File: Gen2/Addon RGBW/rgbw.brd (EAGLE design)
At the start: 59.4 x 48 mm, 33 parts, among them Q1 BUZ11, Q2 BUZ11, Q3 BUZ11, Q4 BUZ11, Q5 BUZ11, Q6 BUZ11, Q7 BUZ11, Q8 BUZ11

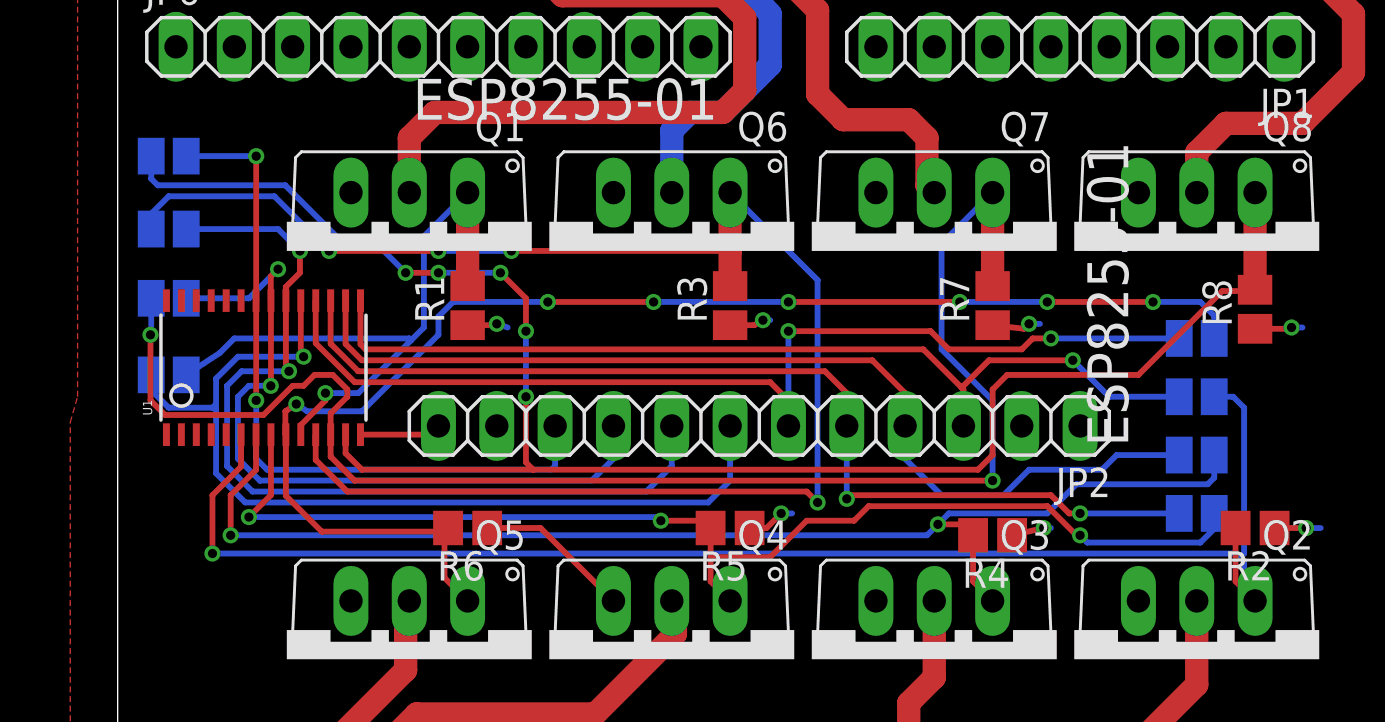
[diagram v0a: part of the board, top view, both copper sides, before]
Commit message: ordner umsortiert und module weiter gemacht
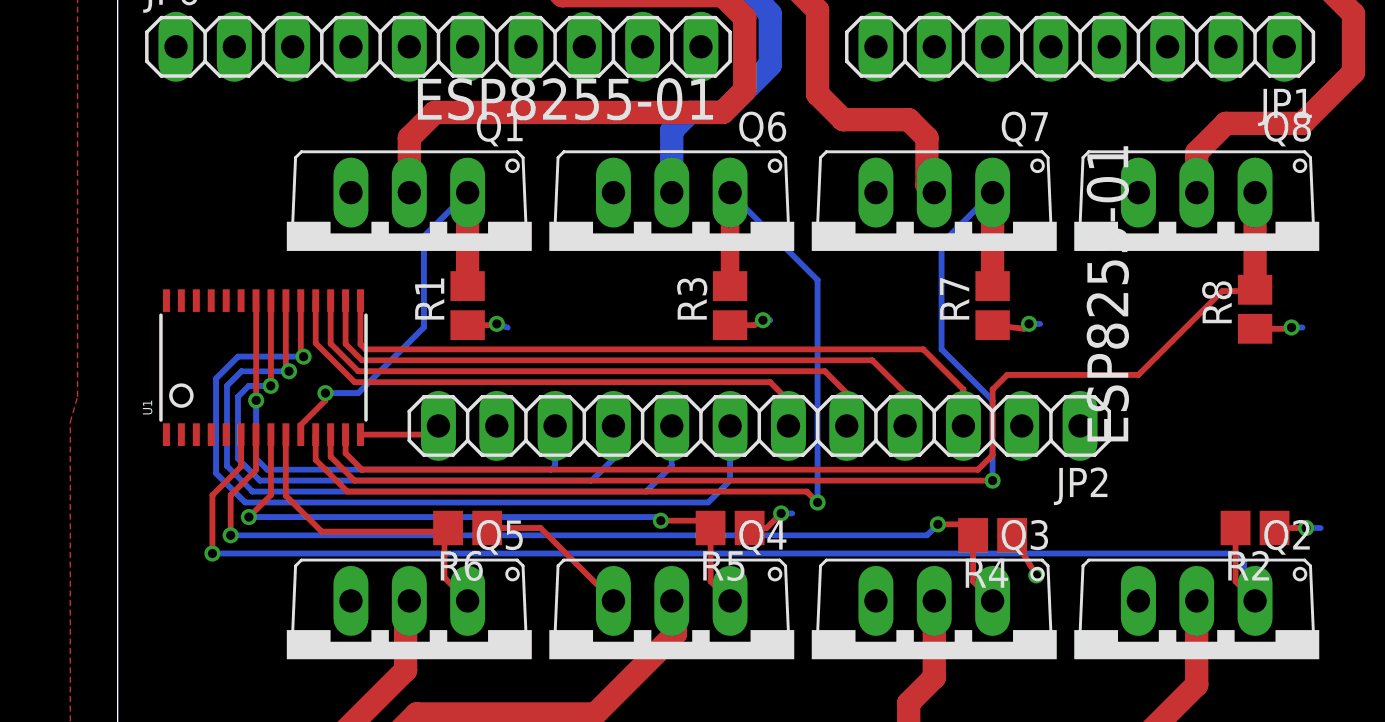
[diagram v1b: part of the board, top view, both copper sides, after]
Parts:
- removed SJ1, SJ2, SJ3, SJ4, SJ5, SJ7, SJ8, SJ9: (no value), jumper:SJ
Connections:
- net LED0: no longer SJ1.2
- net LED1: no longer SJ2.2
- net LED10: no longer SJ3.1
- net LED11: no longer SJ4.1
- net LED12: no longer SJ5.1
- net LED13: no longer SJ8.1
- net LED14: no longer SJ7.1
- net LED15: no longer SJ9.1
- net LED2: no longer SJ3.2
- net LED3: no longer SJ4.2
- net LED4: no longer SJ5.2
- net LED5: no longer SJ8.2
- net LED6: no longer SJ7.2
- net LED7: no longer SJ9.2
- net LED8: no longer SJ1.1
- net LED9: no longer SJ2.1
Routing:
- net LED3: track 59.2 -> 13.9 mm, vias 7 -> 0
- net LED5: track 70.0 -> 42.9 mm, vias 4 -> 1
- net LED7: track 76.9 -> 49.9 mm, vias 5 -> 0
- net LED2: track 52.2 -> 27.8 mm, vias 3 -> 2
- net LED11: track 46.3 -> 24.6 mm, vias 2 -> 0
- net LED10: track 44.8 -> 26.7 mm, vias 2 -> 0
- net LED6: track 65.2 -> 48.7 mm, vias 2 -> 1
- net LED9: track 43.3 -> 28.6 mm
- net LED1: track 54.8 -> 40.9 mm
- net LED8: track 41.2 -> 30.6 mm, vias 1 -> 0
- net LED4: track 28.8 -> 18.5 mm
- net LED15: track 31.3 -> 21.9 mm, vias 2 -> 1
- net LED0: track 64.3 -> 56.2 mm
- net LED13: track 39.4 -> 31.6 mm, vias 2 -> 1
- net LED14: track 32.6 -> 26.6 mm, vias 2 -> 1
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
